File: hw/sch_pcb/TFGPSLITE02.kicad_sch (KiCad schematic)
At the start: 26 parts, among them IC1 CAM-M8Q, J1 SM06B-GHS-TB, J2 SM04B-GHS-TB, M1 HOLE, M2 HOLE, M3 HOLE, M4 HOLE, U1 MIC5504-3.3YM5

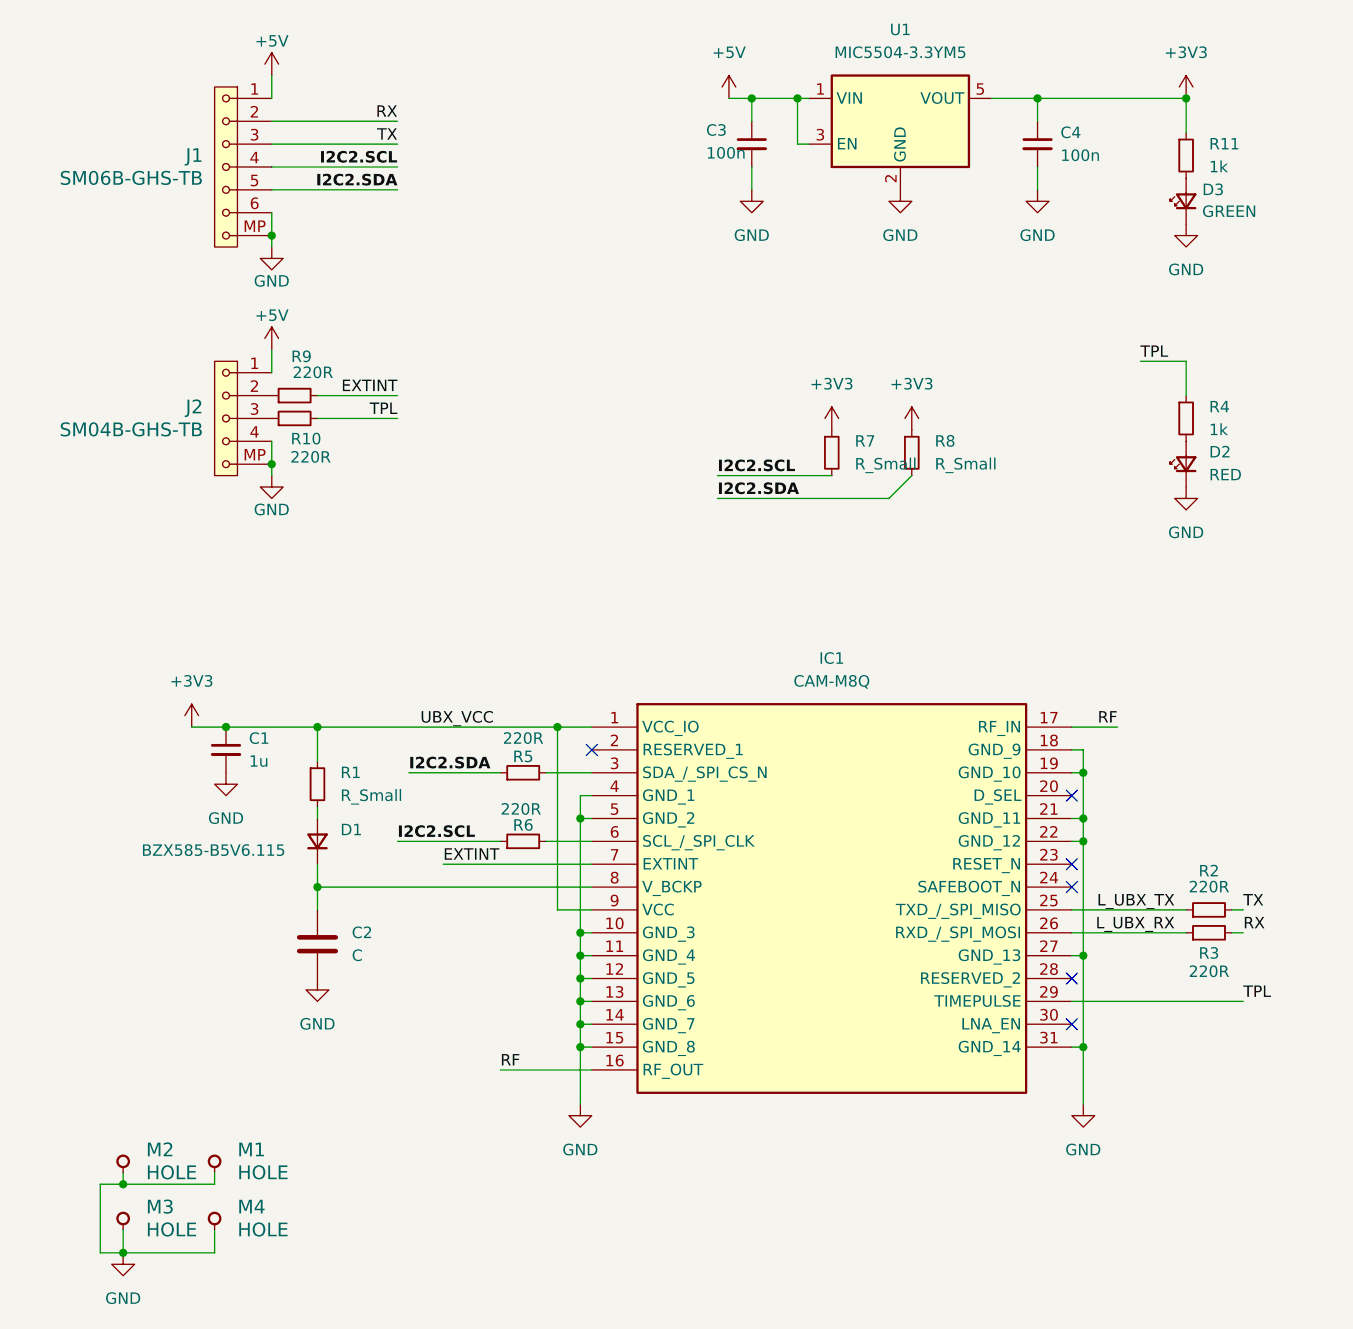
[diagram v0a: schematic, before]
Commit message: Design of TFGPSLITE01
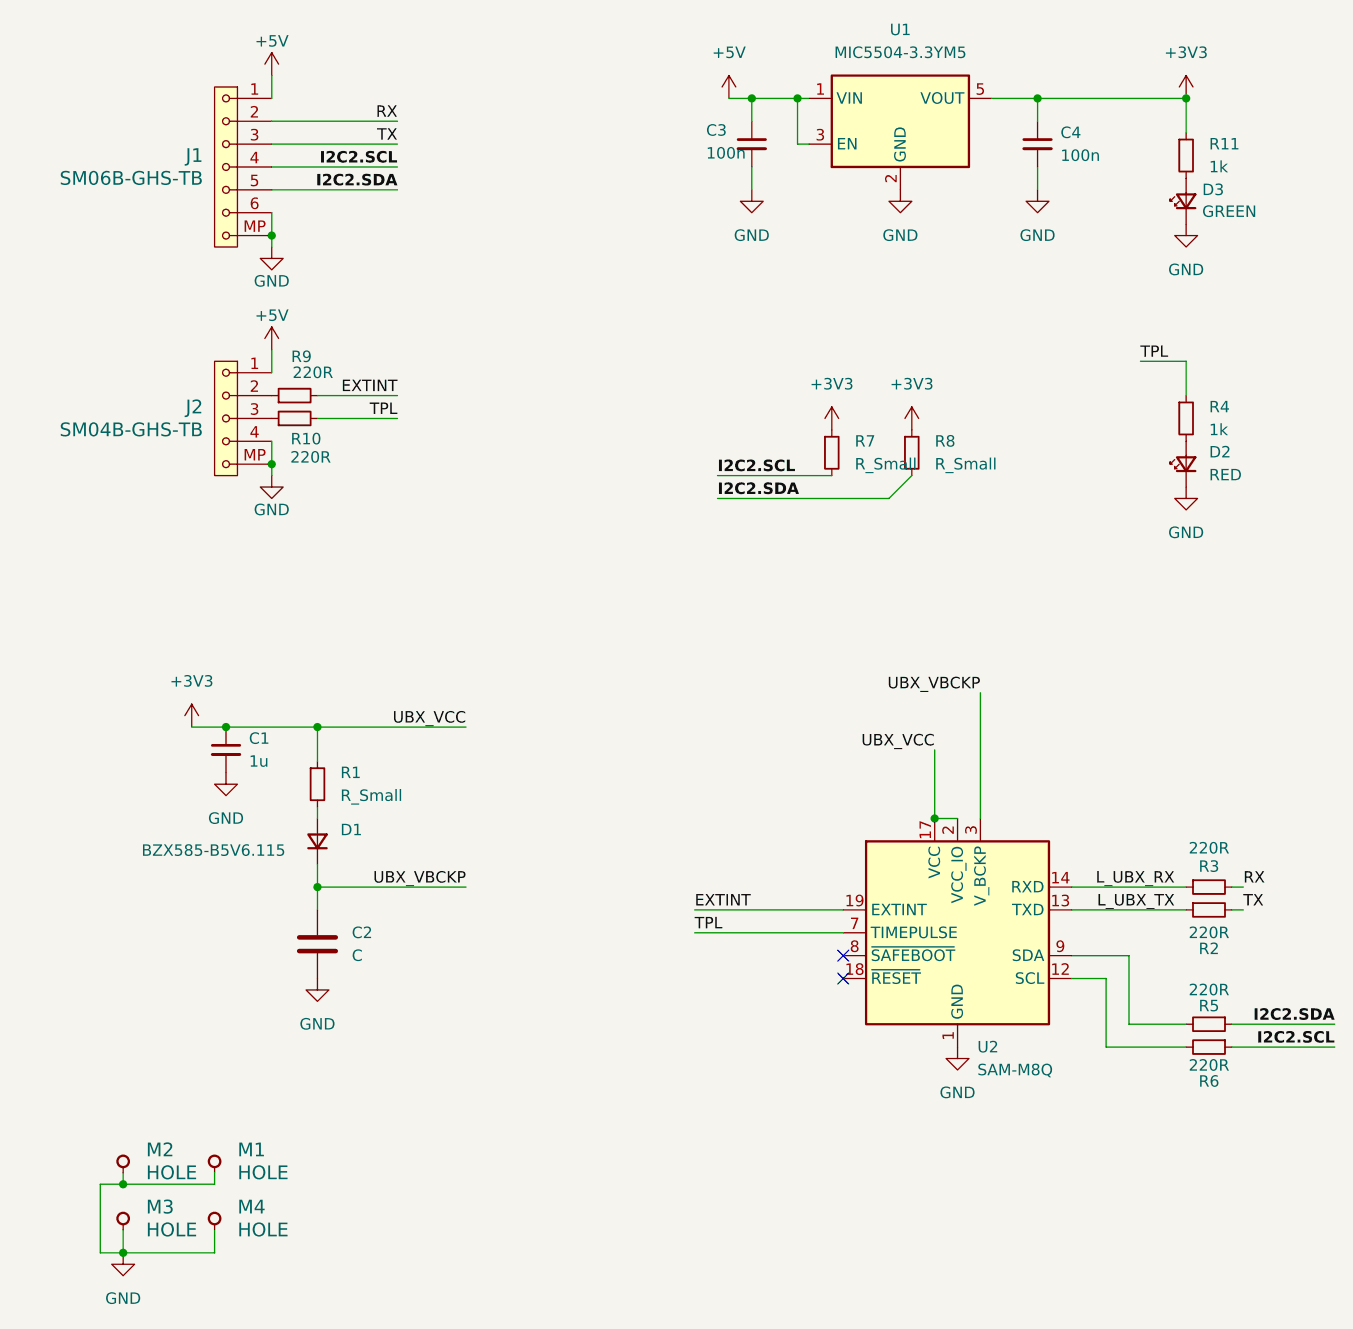
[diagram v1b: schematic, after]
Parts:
- removed IC1: CAM-M8Q, Mlab_IO:CAM-M8Q, symbol MLAB_IO:CAM-M8Q
- added U2: SAM-M8Q, RF_GPS:ublox_SAM-M8Q, symbol RF_GPS:SAM-M8Q
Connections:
- net +3V3: now also U2.17 (VCC), U2.2 (VCC_IO)
- net EXTINT: now also U2.19 (EXTINT)
- net GND: now also U2.1 (GND), U2.10 (GND), U2.11 (GND), U2.15 (GND), U2.16 (GND), U2.20 (GND), U2.4 (GND), U2.5 (GND), U2.6 (GND)
- net L_UBX_RX: now also U2.14 (RXD)
- net L_UBX_TX: now also U2.13 (TXD)
- net TPL: now also U2.7 (TIMEPULSE)
- net UBX_VBCKP: now reaches C2.1, D1.1 (K)
- net UBX_VBCKP: now also U2.3 (V_BCKP)
- net at R6.2: now also U2.12 (SCL)
- net at R5.2: now also U2.9 (SDA)
- no-connect marks 6 -> 2
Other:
- moved on the sheet: R3, R5, R6
